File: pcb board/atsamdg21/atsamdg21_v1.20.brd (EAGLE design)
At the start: 100 x 80 mm, 54 parts, among them IC1 DS3231MZ+, IC2 TPS22810TDBVRQ1, SW1 SPST_TACT-KMR2, U1 ATSAMD21G18A-AU, U2 AP2112K-3.3, U4 RFM69HCW, X1 TSW-105-07-G-S, X2 32.768, X3 microUSB, X4 uFL, X6 TSW-103-08-G-S

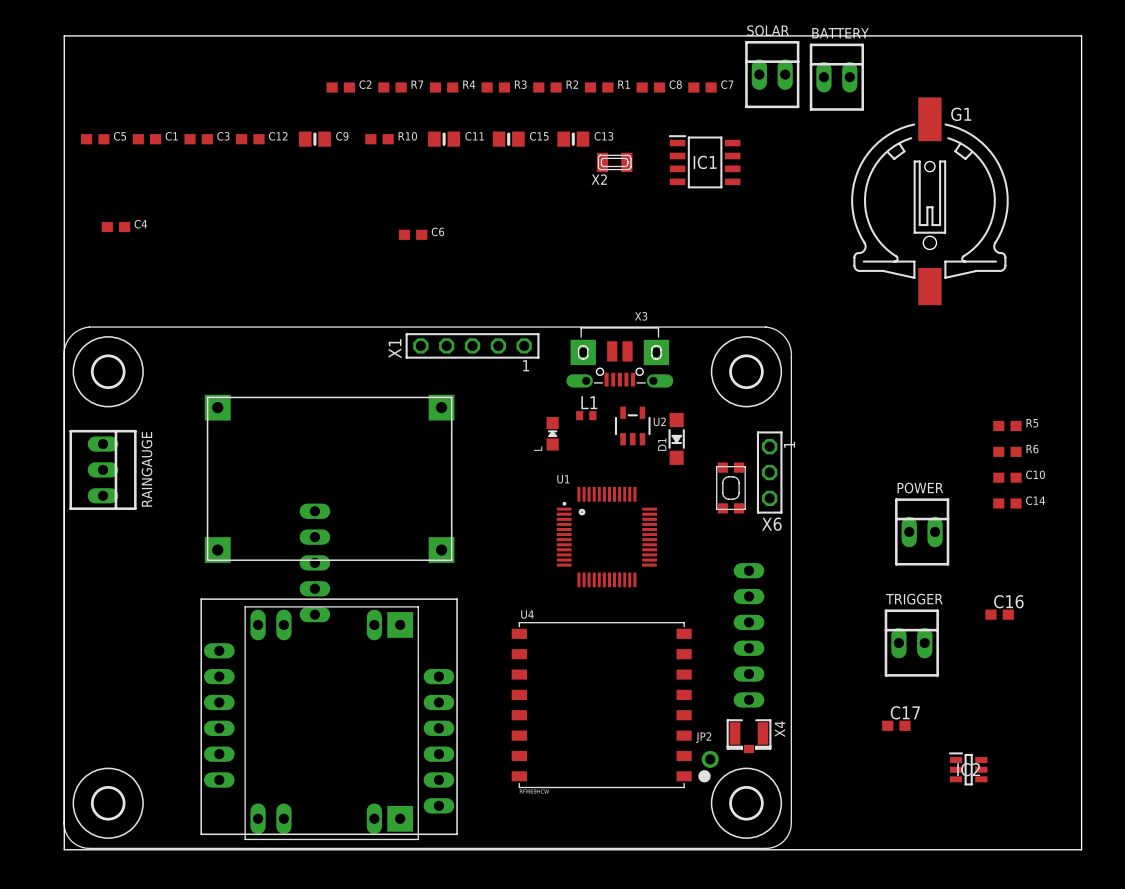
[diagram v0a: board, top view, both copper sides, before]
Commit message: update 05/15
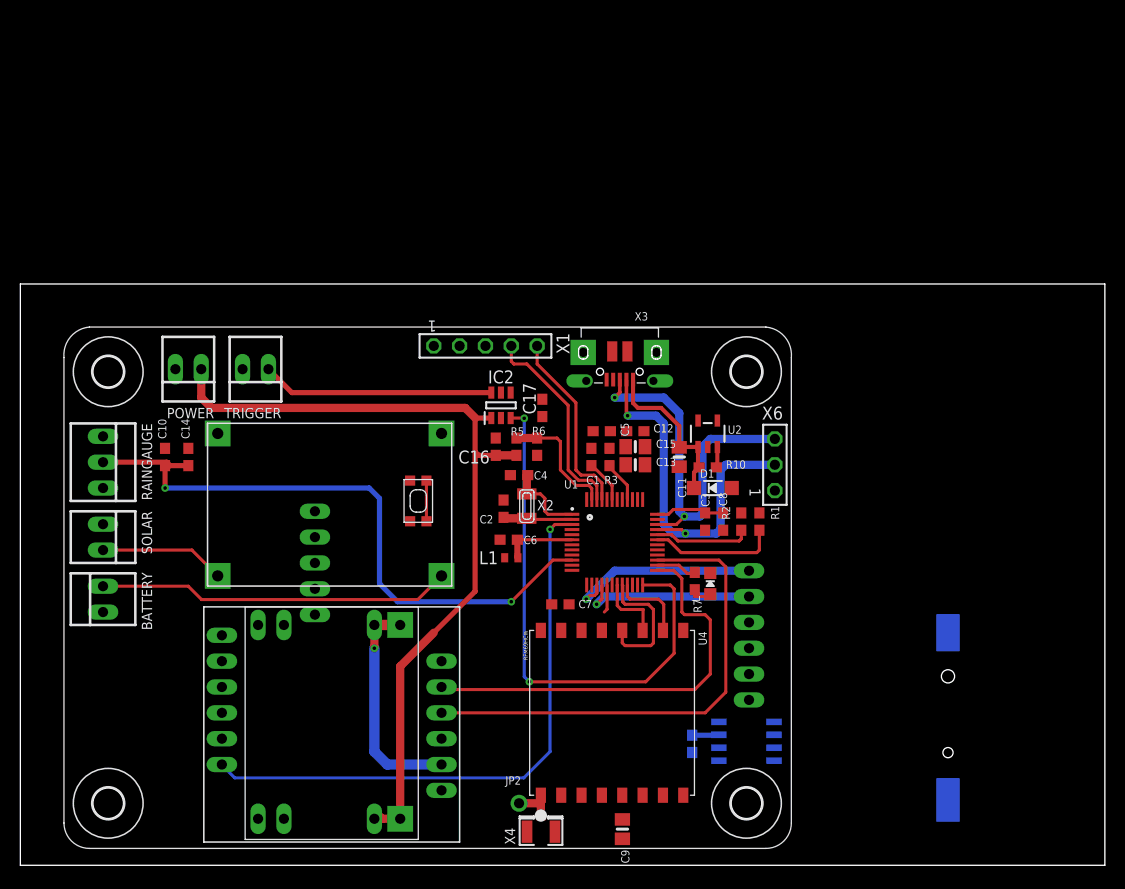
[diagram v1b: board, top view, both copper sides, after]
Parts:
- moved BATTERY 88.5 mm to (3.81, 24.6), turned to 90 degrees
- moved C10 82.8 mm to (9.91, 38.6), turned to 90 degrees
- moved C14 80.6 mm to (12.2, 38.6), turned to 90 degrees
- moved SOLAR 80.0 mm to (3.81, 30.7), turned to 270 degrees
- moved C9 74.2 mm to (54.9, 2.03), turned to 270 degrees
- moved POWER 73.9 mm to (12.2, 47.2), turned to 180 degrees
- moved TRIGGER 69.9 mm to (18.8, 47.2), turned to 180 degrees
- moved R4 69.0 mm to (61.7, 10.4), flipped to the bottom, turned to 270 degrees
- moved C3 62.4 mm to (63.0, 32.3), turned to 270 degrees
- moved IC2 58.3 mm to (42.9, 43.7), turned to 90 degrees
- moved C5 57.5 mm to (52.8, 41.1)
- moved IC1 57.0 mm to (67.1, 10.7), flipped to the bottom, turned to 180 degrees
- moved R7 56.9 mm to (62.0, 26.4), turned to 270 degrees
- moved C1 53.7 mm to (51.8, 38.6), turned to 270 degrees
- moved C7 52.7 mm to (48.8, 24.1)
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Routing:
- net 12VIN: track 0.00 -> 83.2 mm
- net RAIN_G: track 0.00 -> 62.5 mm, vias 0 -> 2
- net A0: track 0.00 -> 58.1 mm, vias 0 -> 1
- net DUETRIG: track 0.00 -> 52.4 mm, vias 0 -> 2
- net D10: track 0.00 -> 48.1 mm
- net D11: track 0.00 -> 42.3 mm
- net USB_D+: track 0.00 -> 38.2 mm, vias 0 -> 2
- net USB_D-: track 0.00 -> 37.8 mm, vias 0 -> 2
- net BATT: track 0.00 -> 34.8 mm
- net N$6: track 0.00 -> 22.9 mm
- net +4V: track 0.00 -> 22.1 mm, vias 0 -> 1
- net SWDIO: track 0.00 -> 20.1 mm
- net TX: track 0.00 -> 19.3 mm, vias 0 -> 1
- net SWCLK: track 0.00 -> 18.5 mm
- net RX: track 0.00 -> 17.4 mm, vias 0 -> 1
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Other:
- board size 100 x 80 mm -> 106.6 x 57.1 mm

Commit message: 05/22 update
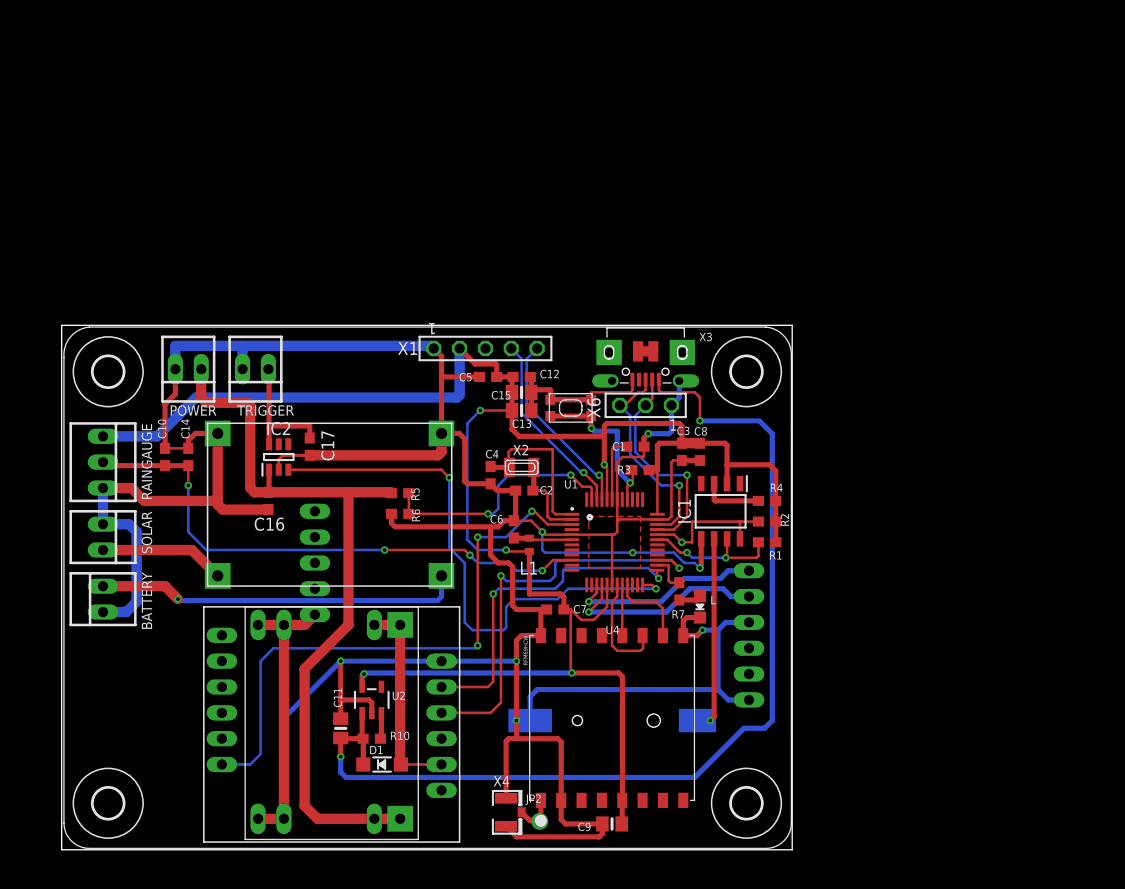
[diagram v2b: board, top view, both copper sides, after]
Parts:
- moved C11 42.6 mm to (27.2, 11.9), turned to 90 degrees
- moved R10 42.4 mm to (30.2, 10.9)
- moved D1 42.4 mm to (31.2, 8.38)
- moved U2 42.1 mm to (30.2, 14.7)
- moved G1 27.7 mm to (59.9, 12.7), turned to 270 degrees
- moved R4 25.0 mm to (69.1, 34.3), flipped to the top, turned to 0 degrees
- moved C17 23.2 mm to (24.1, 39.6), turned to 270 degrees
- moved C16 23.0 mm to (20.1, 34.3), turned to 90 degrees
- moved IC1 22.7 mm to (64.5, 33.3), flipped to the top, turned to 270 degrees
- moved IC2 22.4 mm to (21.1, 38.6)
- moved SW1 17.6 mm to (49.8, 43.4), turned to 180 degrees
- moved R6 15.0 mm to (33.0, 33.0), turned to 180 degrees
- moved X6 14.0 mm to (57.1, 43.7), turned to 0 degrees
- moved C13 12.4 mm to (45.0, 43.2)
- moved C12 12.4 mm to (45.0, 46.5)
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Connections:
- removed net N$3: R3.2, U1.40
- removed net N$8: C17.1
- net !RESET: now also R3.2, U1.40
- net N$6: now also C17.1
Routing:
- net GND: track 0.00 -> 412.4 mm, vias 0 -> 8
- net +3V3: track 9.57 -> 197.1 mm, vias 0 -> 5
- net VBUS: track 16.6 -> 99.1 mm, vias 0 -> 2
- net N$2: track 0.00 -> 19.3 mm, vias 0 -> 1
- net USB_D+: track 38.2 -> 21.0 mm, vias 2 -> 1
- net USB_D-: track 37.8 -> 21.3 mm, vias 2 -> 1
- net !RESET: track 4.00 -> 16.7 mm, vias 0 -> 2
- net VOLT_SENS: track 12.2 -> 24.6 mm, vias 0 -> 2
- net N$6: track 22.9 -> 12.7 mm
- net D11: track 42.3 -> 33.1 mm, vias 0 -> 2
- net 12VIN: track 83.2 -> 74.9 mm
- net N$7: track 7.90 -> 16.0 mm
- net SCK: track 12.8 -> 4.97 mm
- net RAIN_G: track 62.5 -> 54.8 mm, vias 2 -> 4
- net D10: track 48.1 -> 40.8 mm, vias 0 -> 2
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- added copper zone on layer 1, net GND
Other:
- board size 106.6 x 57.1 mm -> 71.8 x 51.6 mm
